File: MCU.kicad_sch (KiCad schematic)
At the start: 30 parts, among them J1 HSEC8-150-01-X-RA-X, J17 Conn_02x30_Counter_Clockwise, J2 Barrel_Jack_MountingPin, J22 Conn_01x02, J23 Conn_01x02, J4 Conn_02x30_Counter_Clockwise, J6 Conn_01x02, U3 LMR36510ADDA

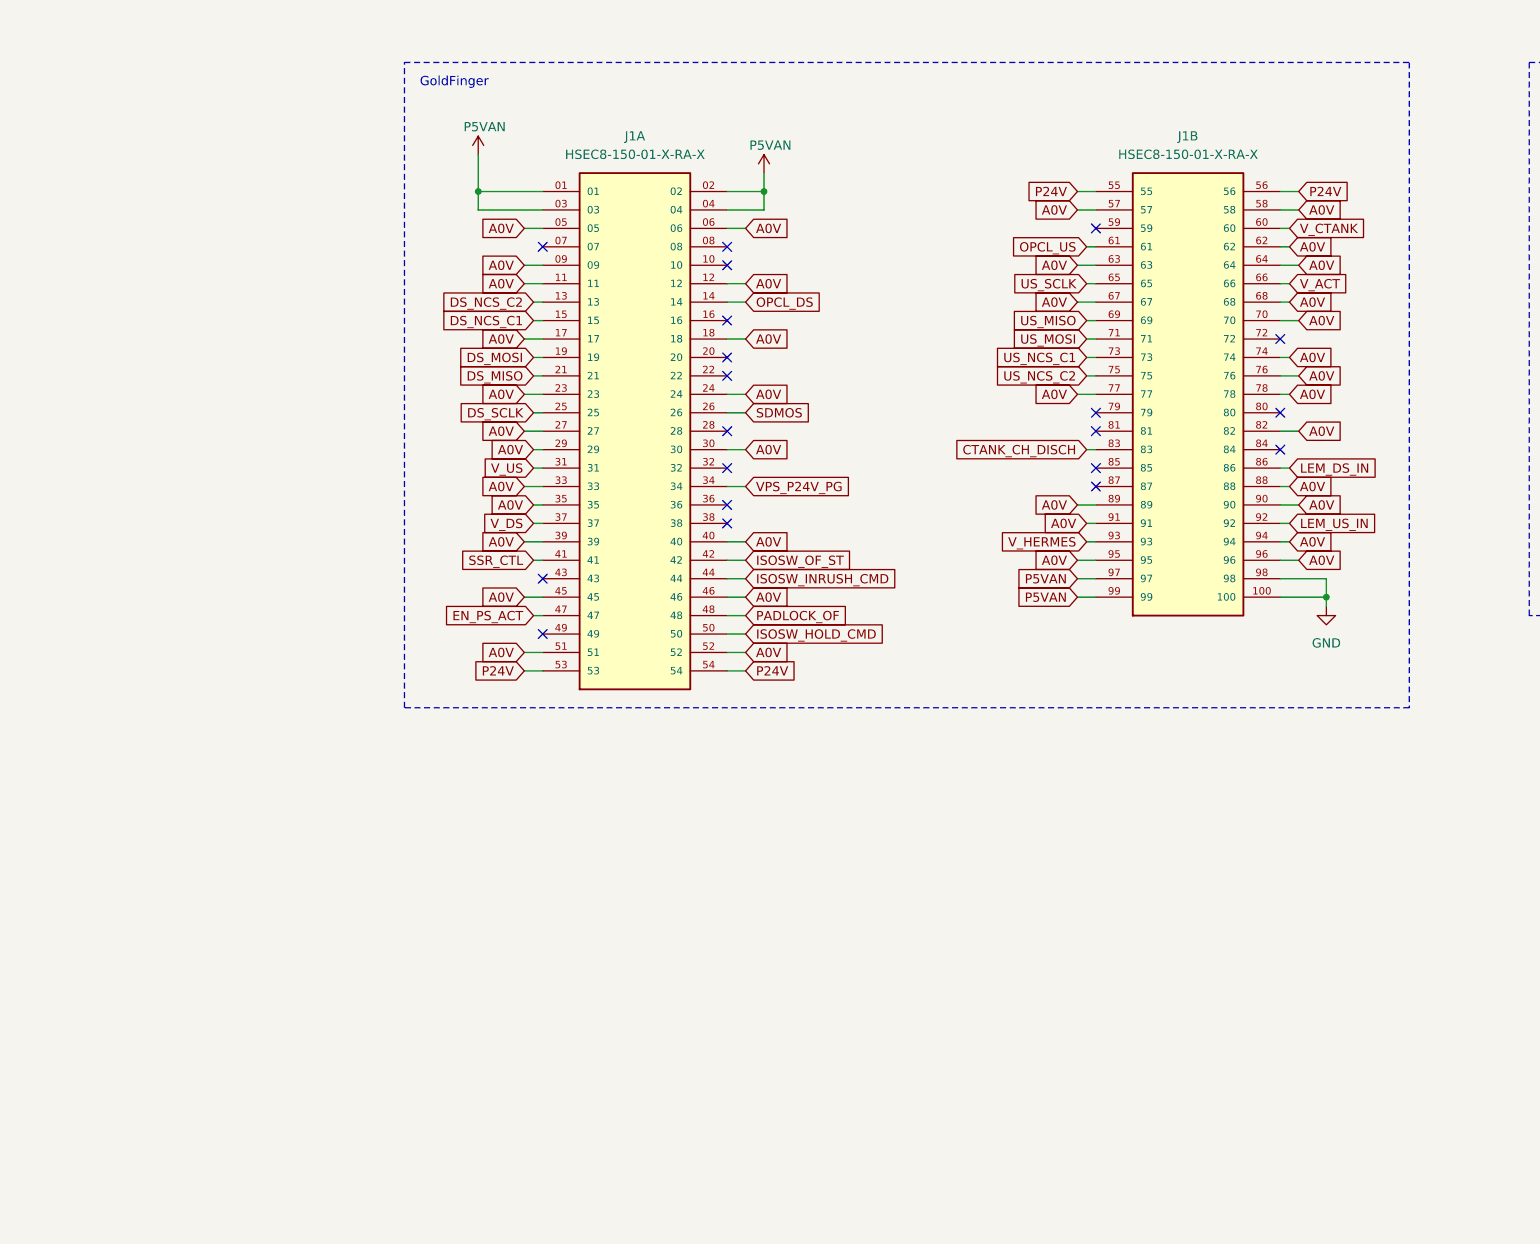
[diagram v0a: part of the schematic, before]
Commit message: Go vertical + BOM
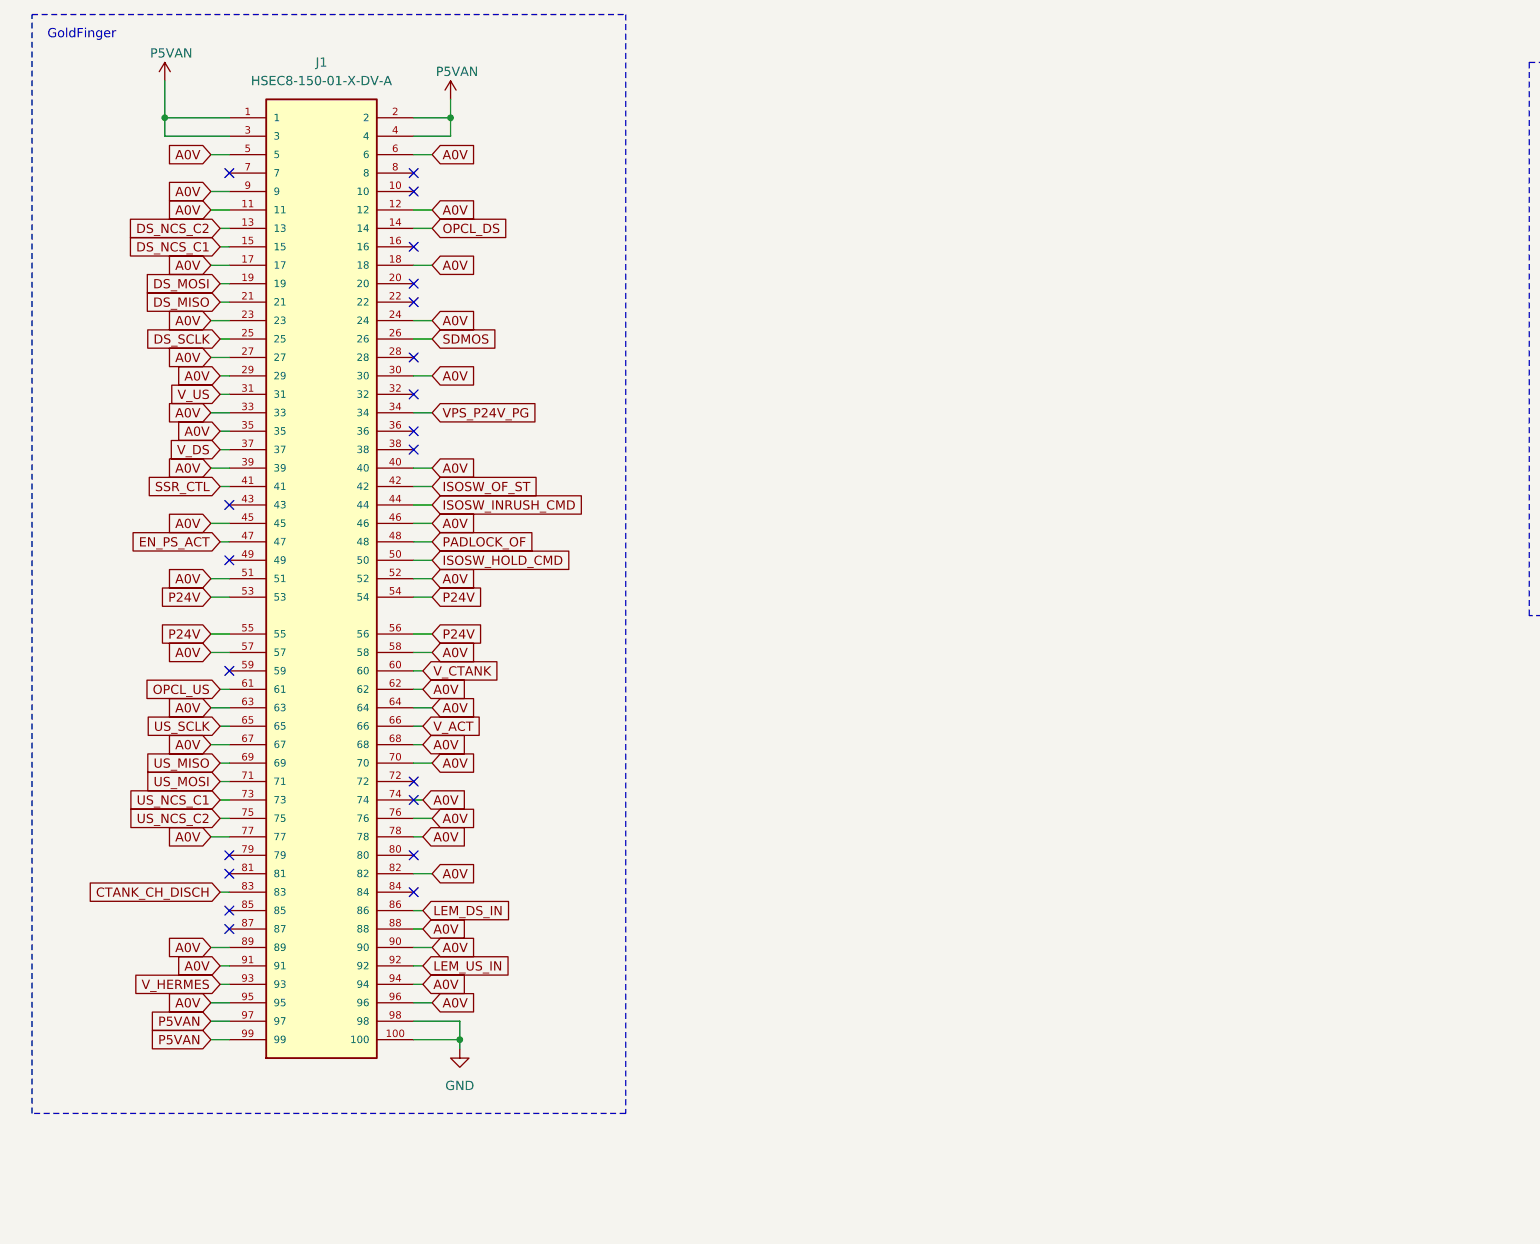
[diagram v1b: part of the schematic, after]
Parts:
- removed J1: HSEC8-150-01-X-RA-X, kicad_jlcpcb_hil_mcu_ep2:SAMTEC_HSEC8-150-01-X-RA-X, symbol HSEC8-150-01-X-RA-X:HSEC8-150-01-X-RA-X
- added J1: HSEC8-150-01-X-DV-A, Connector_Samtec_HSEC8:Samtec_HSEC8-150-01-X-DV-A_2x50_P0.8mm_Pol27_Socket_AlignmentPins, symbol HSEC8-150-01-X-DV-A:HSEC8-150-01-X-DV-A
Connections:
- net CTANK_CH_DISCH: now also J1.83
- net DS_MISO: now also J1.21
- net DS_MOSI: now also J1.19
- net DS_NCS_C1: now also J1.15
- net DS_NCS_C2: now also J1.13
- net DS_SCLK: now also J1.25
- net EN_PS_ACT: now also J1.47
- net GND: now also J1.100, J1.11, J1.12, J1.17, J1.18, J1.23, J1.24, J1.27, J1.29, J1.30, J1.33, J1.35, J1.39, J1.40, J1.45, J1.46, J1.5, J1.51, J1.52, J1.57, J1.58, J1.6, J1.62, J1.63, J1.64, J1.67, J1.68, J1.70, J1.74, J1.76, J1.77, J1.78, J1.82, J1.88, J1.89, J1.9, J1.90, J1.91, J1.94, J1.95, J1.96, J1.98
- net ISOSW_HOLD_CMD: now also J1.50
- net ISOSW_INRUSH_CMD: now also J1.44
- net ISOSW_OF_ST: now also J1.42
- net LEM_DS_IN: now also J1.86
- net LEM_US_IN: now also J1.92
- net OPCL_DS: now also J1.14
- net OPCL_US: now also J1.61
- net P24V: now also J1.53, J1.54, J1.55, J1.56
- net P5VAN: now also J1.1, J1.2, J1.3, J1.4, J1.97, J1.99
- net PADLOCK_OF: now also J1.48
- net SDMOS: now also J1.26
- net SSR_CTL: now also J1.41
- net US_MISO: now also J1.69
- net US_MOSI: now also J1.71
- net US_NCS_C1: now also J1.73
- net US_NCS_C2: now also J1.75
- net US_SCLK: now also J1.65
- net VPS_P24V_PG: now also J1.34
- net V_ACT: now also J1.66
- net V_CTANK: now also J1.60
- net V_DS: now also J1.37
- net V_HERMES: now also J1.93
- net V_US: now also J1.31
- no-connect marks 27 -> 28
